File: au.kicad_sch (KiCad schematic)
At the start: 16 parts, among them Q1 SUM110P06-08L, Q2 2N7002, Q3 2N7002

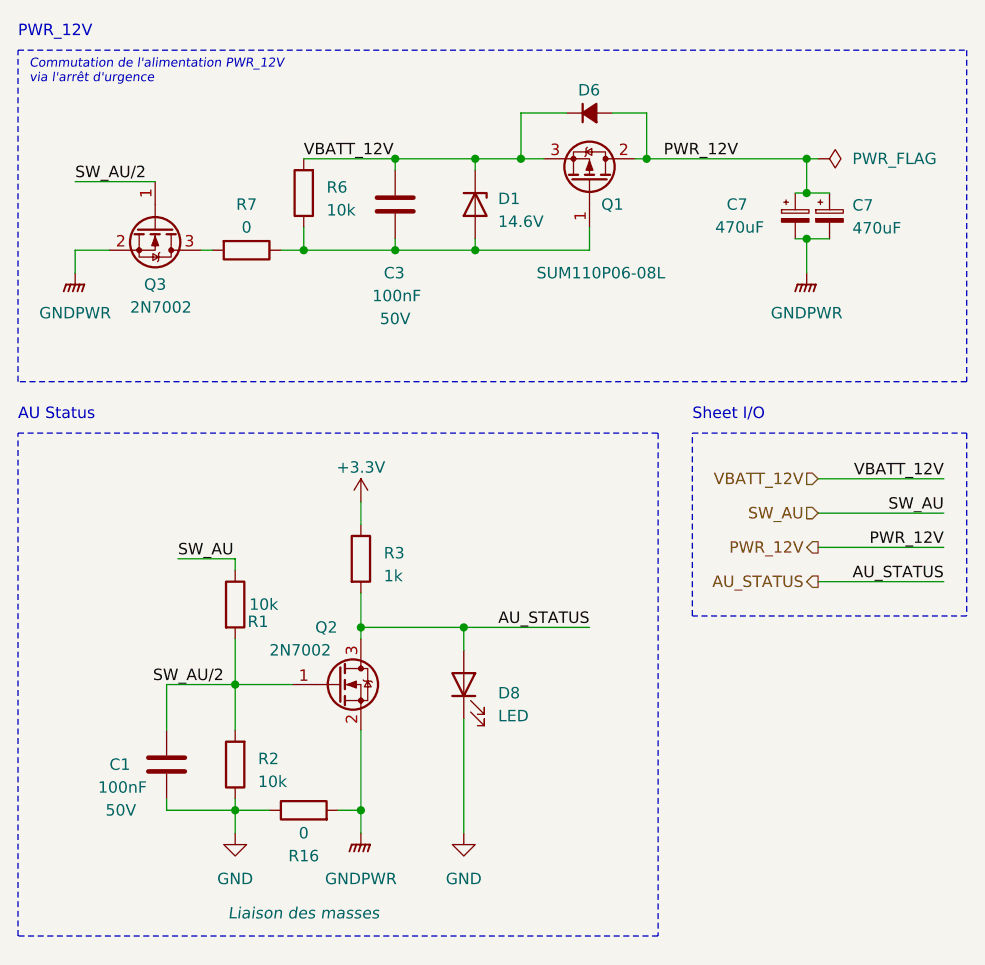
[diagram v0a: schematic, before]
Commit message: Schematics finished, reanotated sch
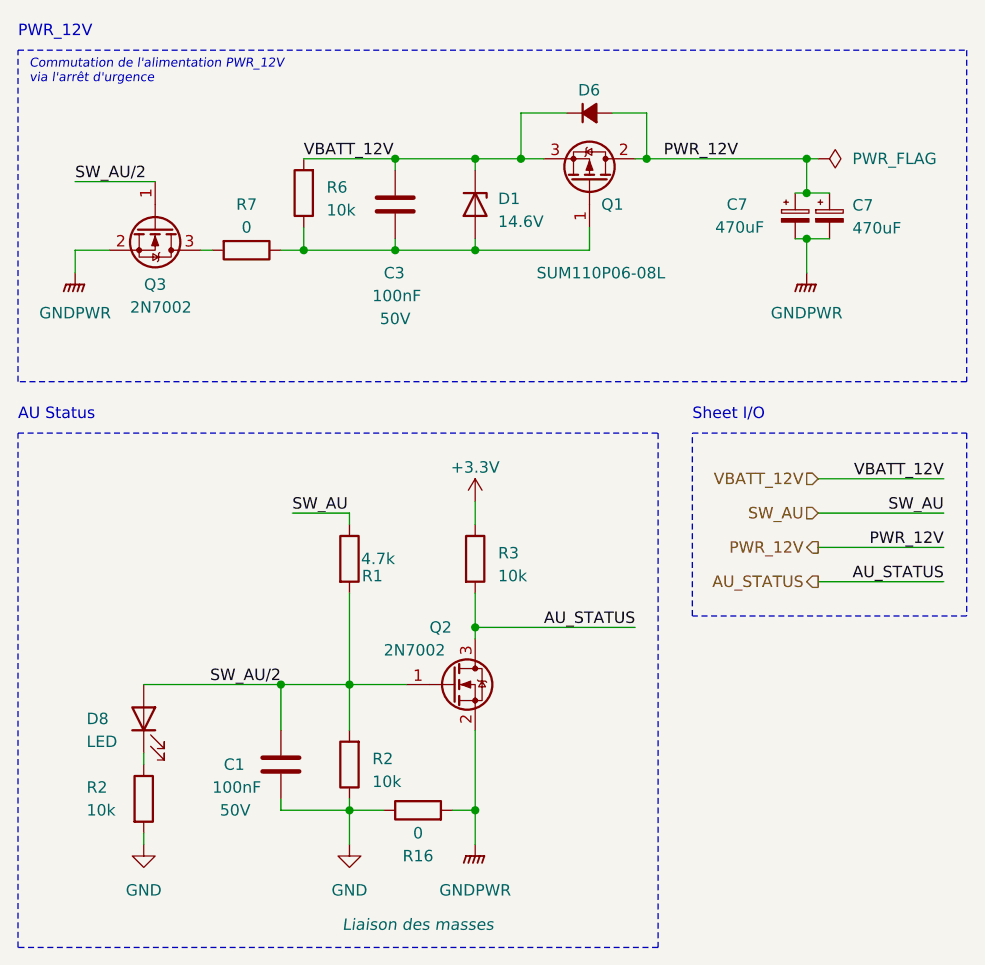
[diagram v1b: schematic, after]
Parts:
- added R2: 10k, Resistor_SMD:R_0603_1608Metric, symbol Device:R
- R1: value 10k -> 4.7k; footprint Resistor_SMD:R_0201_0603Metric -> Resistor_SMD:R_0603_1608Metric
- R3: value 1k -> 10k
- R6, R7: footprint Resistor_SMD:R_0201_0603Metric -> Resistor_SMD:R_0603_1608Metric
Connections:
- net AU_STATUS: no longer D8.2 (A)
- net GND: now also R2.2; no longer D8.1 (K)
- net SW_AU/2: now also D8.2 (A)
- new net: D8.1 (K), R2.1
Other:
- moved on the sheet: C1, D8, Q2, R1, R16, R2, R3
